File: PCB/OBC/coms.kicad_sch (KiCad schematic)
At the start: 25 parts, among them U4 STM32F405RGTx

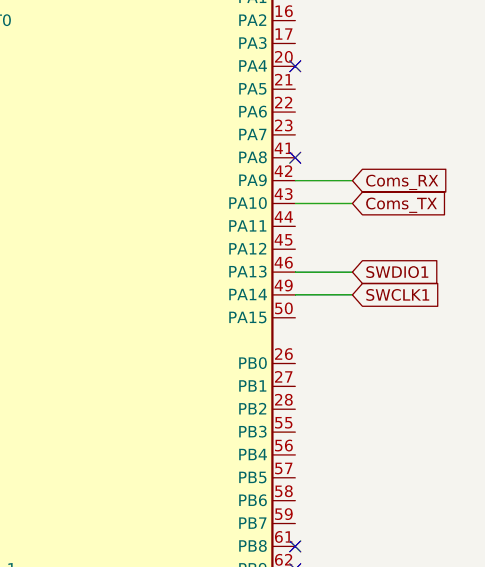
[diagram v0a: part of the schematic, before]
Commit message: New
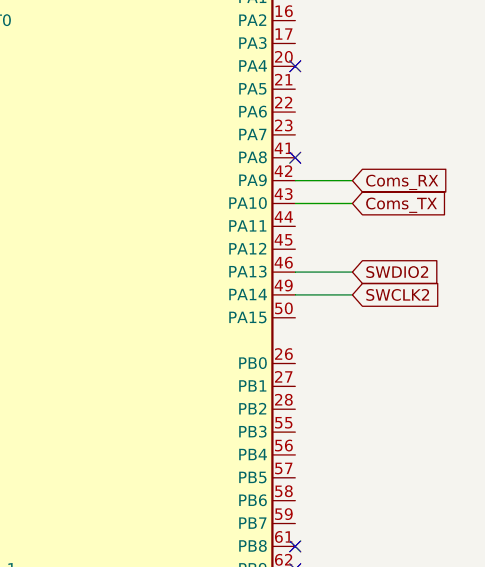
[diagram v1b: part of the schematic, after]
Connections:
- net SWCLK1 renamed SWCLK2
- net SWDIO1 renamed SWDIO2
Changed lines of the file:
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@@
 		)
 	)
-	(global_label "SWCLK1"
+	(global_label "SWCLK2"
 		(shape input)
 		(at 143.51 83.82 0)
@@
 		)
 	)
-	(global_label "SWDIO1"
+	(global_label "SWDIO2"
 		(shape input)
 		(at 143.51 81.28 0)
